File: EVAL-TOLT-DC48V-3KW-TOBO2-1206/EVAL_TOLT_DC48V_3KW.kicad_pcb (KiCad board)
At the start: 6 copper layers, 170 x 120 mm, 148 parts, among them IC1 LM5013QDDARQ1, J1 V_BAT+, J12 Direction Switch, J2 V_BAT-, J3 EXT/ITN 12V, J4 +12V_EXT, J5 +5V_EXT, M1 MountingHole_3.2mm_M3_DIN965, M2 MountingHole_3.2mm_M3_DIN965, M3 MountingHole_3.2mm_M3_DIN965, M4 MountingHole_3.2mm_M3_DIN965, Q1 IAUS300N10S5N015TATMA1, Q4 IAUS300N10S5N015TATMA1, Q7 IRLML6346, Q8 IRLML6346, U11 LMV331, U12 PCN10-32S-2.54DSA72, U13 SN74LVC2G74DCUR, U3 2EDL8x24G, U4 NL27WZ08USG

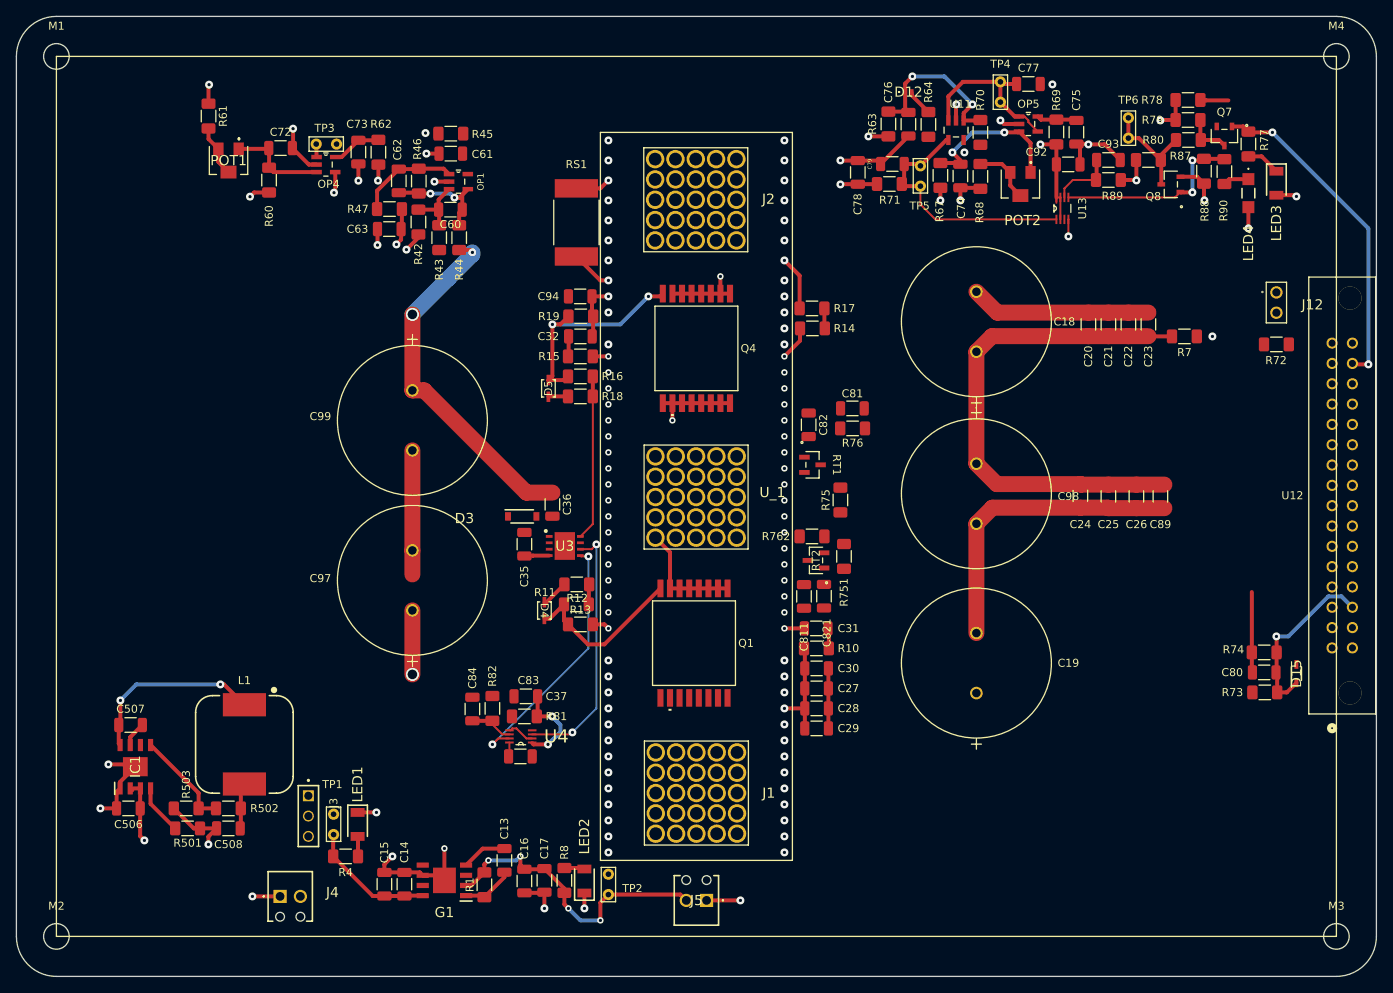
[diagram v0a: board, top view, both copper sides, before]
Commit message: v08112024
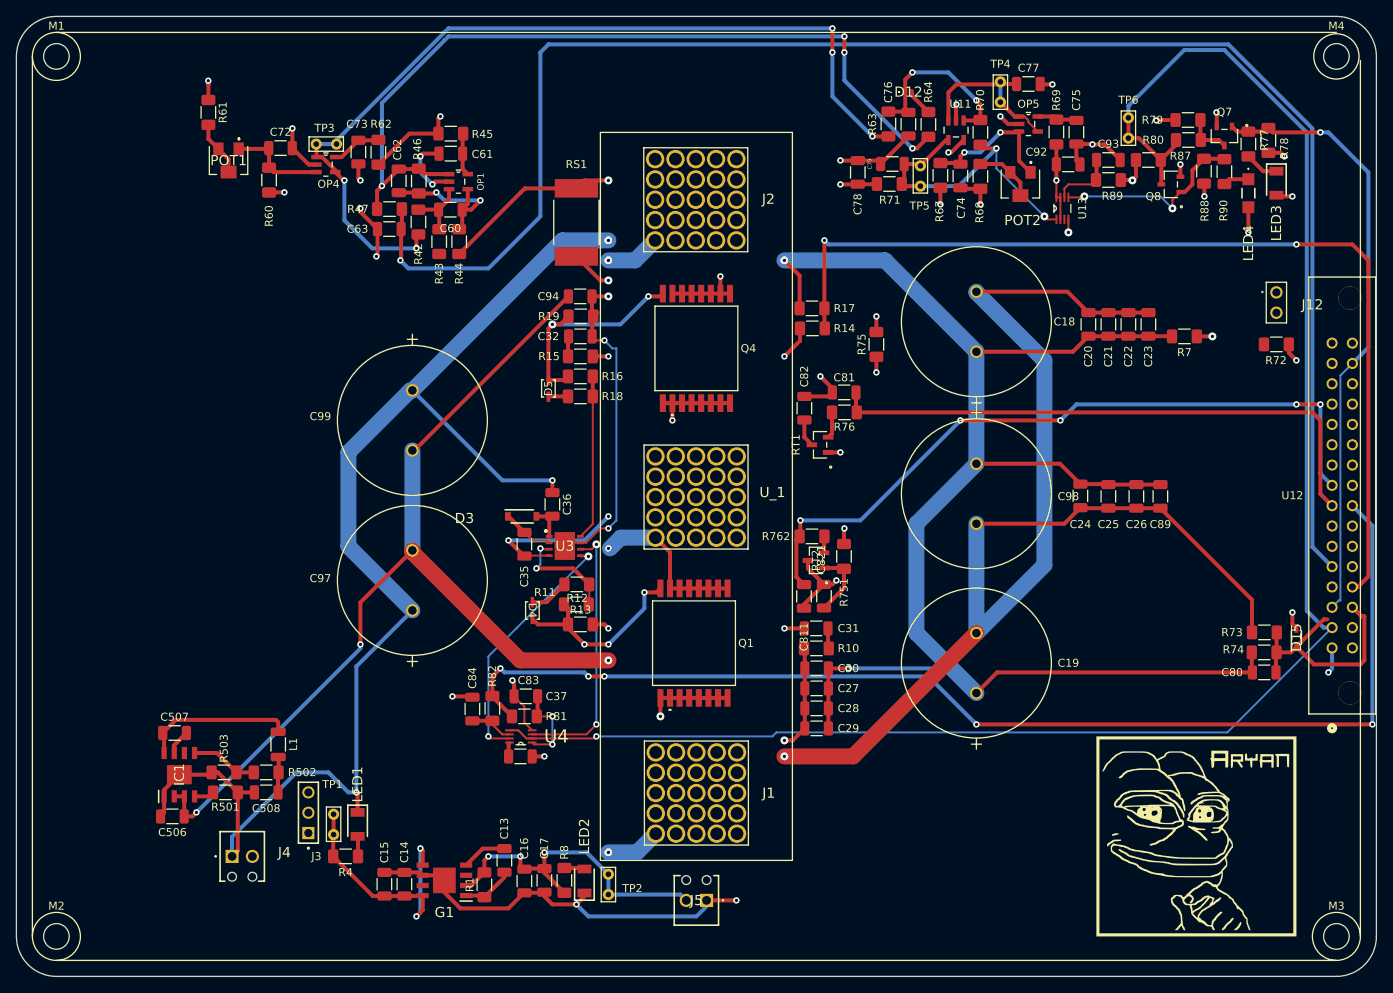
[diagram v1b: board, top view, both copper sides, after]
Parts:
- added G***: LOGO, 1206-Infineon-Library:Aryan-Pepe-Logo, F.Cu at (227.5, 132.5)
- J3: footprint just-footprints:SAMTEC_TSW-103-08-L-S -> just-footprints:SAMTEC_HTSW-103-XX-X-S
- L1: footprint Misc-Footprints:L1 -> Inductor_SMD:L_1206_3216Metric
- moved R75 20.0 mm to (187.5, 71.0)
- moved R78 11.2 mm to (236.5, 45.5), turned to 90 degrees
- moved J4 7.81 mm to (107.0, 135.0)
- moved R73 7.50 mm to (236.0, 107.0)
- moved R503 6.53 mm to (106.0, 124.5)
- moved C508 6.52 mm to (111.2, 127.0)
- moved R501 6.52 mm to (106.1, 127.0)
- moved R502 6.52 mm to (111.2, 124.5)
- moved C506 5.59 mm to (99.5, 130.0)
- moved C507 5.59 mm to (99.8, 119.6)
- moved IC1 5.59 mm to (100.4, 124.8)
- moved D15 4.50 mm to (240.0, 107.7)
- moved L1 4.22 mm to (112.7, 121.0), turned to -90 degrees
- moved RT1 2.67 mm to (180.5, 83.5), turned to 90 degrees
- moved C81 2.25 mm to (183.5, 77.0)
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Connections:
- C62 pad 2: Net-(OP1-OUT) -> I_PHASE_U
- OP1 pad 1: Net-(OP1-OUT) -> I_PHASE_U
- R46 pad 2: Net-(OP1-OUT) -> I_PHASE_U
- R47 pad 1: Net-(OP1-OUT) -> I_PHASE_U
- R73 pad 2: V_BATT+ -> V_BAT+
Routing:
- net V_BAT-: track 171.9 -> 394.3 mm, vias 22 -> 7
- net V_BAT+: track 97.0 -> 311.0 mm, vias 27 -> 7
- net SD: track 17.5 -> 217.8 mm, vias 0 -> 1
- net I_SNS_PHASE_U: track 4.70 -> 205.0 mm
- net U-L: track 0.18 -> 147.7 mm, vias 0 -> 5
- net BEMF_PHASE_U: track 2.52 -> 122.1 mm, vias 0 -> 2
- net I_PHASE_U: track 0.00 -> 104.5 mm, vias 0 -> 4
- net OFFSET: track 9.29 -> 112.1 mm, vias 3 -> 5
- net Net-(C811-Pad2): track 0.00 -> 90.4 mm, vias 0 -> 5
- net Net-(C81-Pad2): track 0.00 -> 72.2 mm
- net GNDS: track 25.0 -> 76.7 mm, vias 5 -> 8
- net /U-Phase/U_CS+: track 21.8 -> 55.4 mm, vias 10 -> 5
- net /Power Board Connector/DR_EN: track 44.9 -> 76.3 mm, vias 2 -> 1
- net GND: track 54.3 -> 80.1 mm, vias 16 -> 22
- net /U-Phase/U: track 37.9 -> 61.7 mm, vias 37 -> 8
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- added copper zone on In4.Cu, net GNDS
- removed copper zone on In1.Cu, net GNDS
- removed copper zone on In4.Cu, net OFFSET
